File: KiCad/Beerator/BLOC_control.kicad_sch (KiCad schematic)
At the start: 10 parts, among them Y301 16MHz

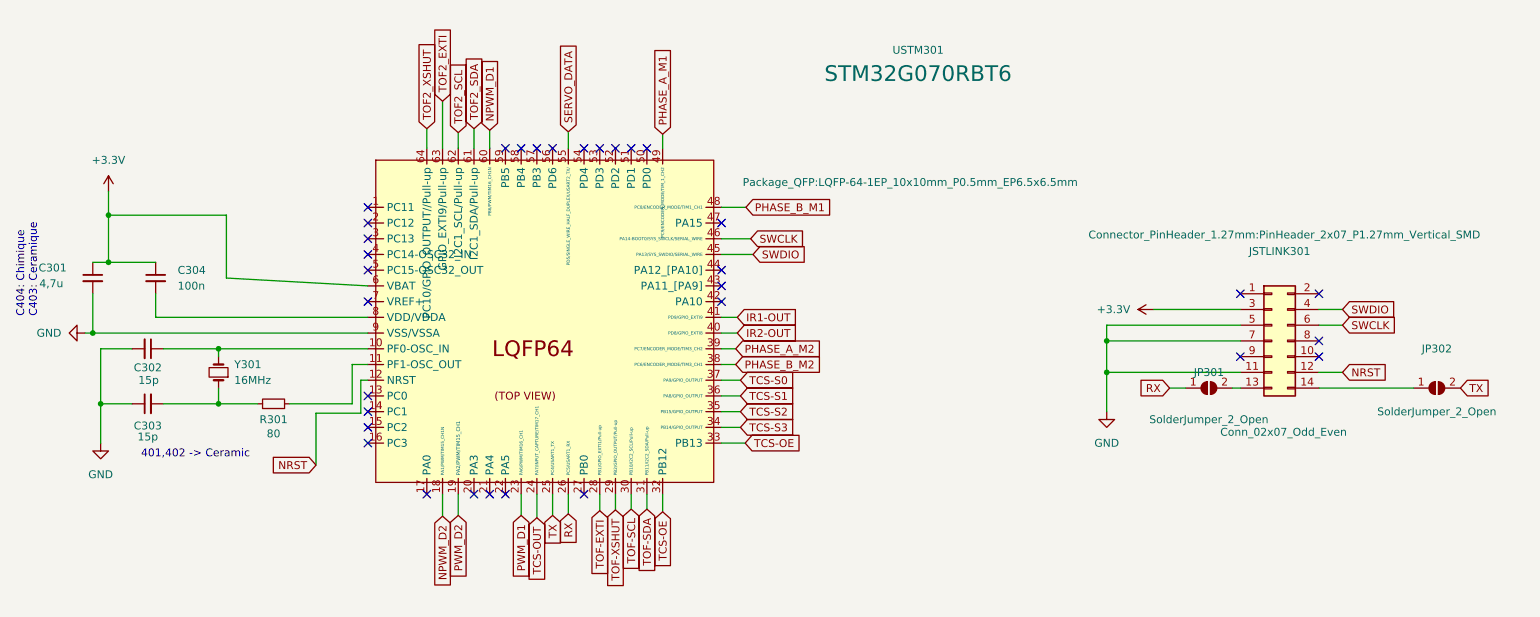
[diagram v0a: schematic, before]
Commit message: pcb_v2
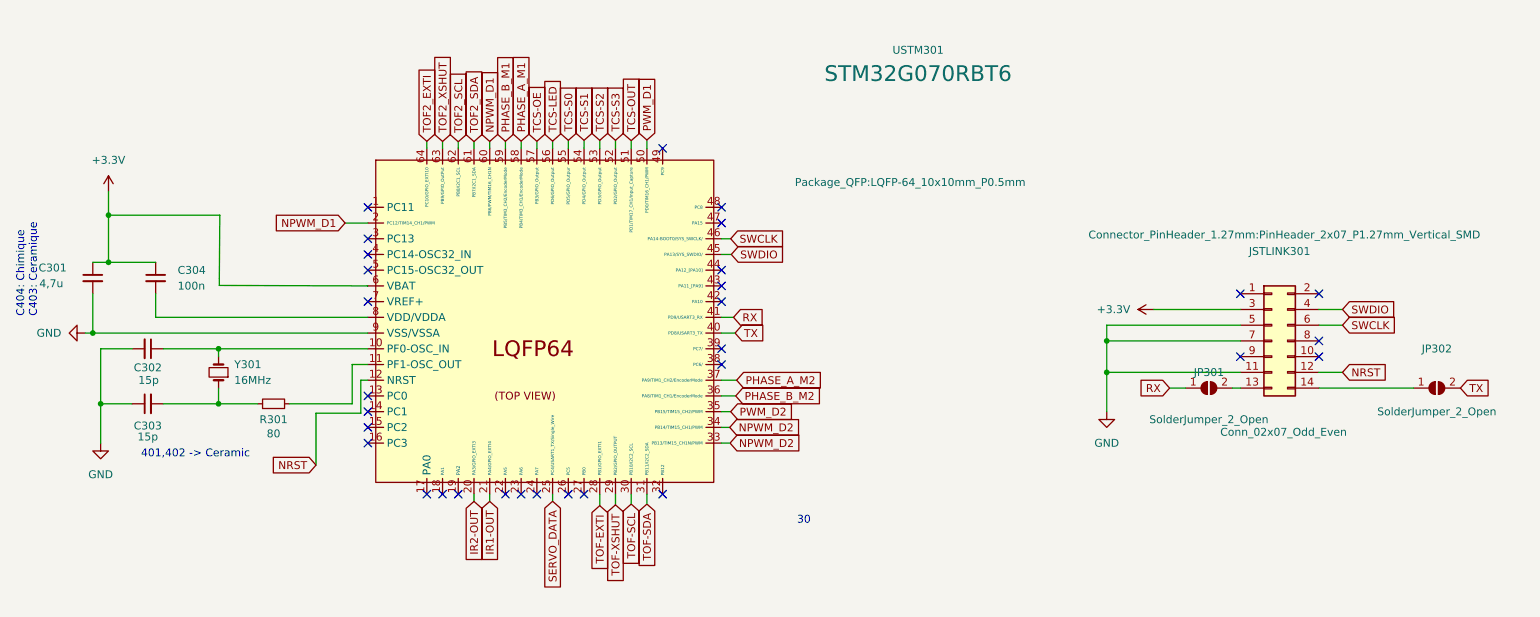
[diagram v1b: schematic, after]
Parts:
- USTM301: footprint Package_QFP:LQFP-64-1EP_10x10mm_P0.5mm_EP6.5x6.5mm -> Package_QFP:LQFP-64_10x10mm_P0.5mm
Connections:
- net IR1-OUT: now also USTM301.21 (PA4/GPIO_EXTI4); no longer USTM301.41 (PD9/GPIO_EXTI9)
- net IR2-OUT: now also USTM301.20 (PA3/GPIO_EXTI3); no longer USTM301.40 (PD8/GPIO_EXTI8)
- net NPWM_D1: now also USTM301.2 (PC12/TIM14_CH1/PWM)
- net NPWM_D2: now also USTM301.33 (PB13/TIM15_CH1N/PWM), USTM301.34 (PB14/TIM15_CH1/PWM); no longer USTM301.18 (PA1/PWM/TIM15_CH1N)
- net PHASE_A_M1: now also USTM301.58 (PB4/TIM3_CH1/EncoderMode); no longer USTM301.49 (PC9/ENCODER_MODE/TIM_1_CH2)
- net PHASE_A_M2: now also USTM301.37 (PA9/TIM1_CH2/EncoderMode); no longer USTM301.39 (PC7/ENCODER_MODE/TIM3_CH2)
- net PHASE_B_M1: now also USTM301.59 (PB5/TIM3_CH2/EncoderMode); no longer USTM301.48 (PC8/ENCODER_MODE/TIM1_CH1)
- net PHASE_B_M2: now also USTM301.36 (PA8/TIM1_CH1/EncoderMode); no longer USTM301.38 (PC6/ENCODER_MODE/TIM3_CH1)
- net PWM_D1: now also USTM301.50 (PD0/TIM16_CH1/PWM); no longer USTM301.23 (PA6/PWM/TIM16_CH1)
- net PWM_D2: now also USTM301.35 (PB15/TIM15_CH2/PWM); no longer USTM301.19 (PA2/PWM/TIM15_CH1)
- net RX: now also USTM301.41 (PD9/USART3_RX); no longer USTM301.26 (PC5/USART1_RX)
- net SERVO_DATA: now also USTM301.25 (PC4/USART1_TX/Single_Wire); no longer USTM301.55 (PD5/SINGLE_WIRE_HALF_DUPLEX/USART2_TX/)
- net TCS-OE: now also USTM301.57 (PB3/GPIO_Output); no longer USTM301.32 (PB12), USTM301.33 (PB13)
- net TCS-OUT: now also USTM301.51 (PD1/TIM17_CH1/Input_Capture); no longer USTM301.24 (PA7/INPUT_CAPTURE/TIM17_CH1)
- net TCS-S0: now also USTM301.55 (PD5/GPIO_Outpur); no longer USTM301.37 (PA9/GPIO_OUTPUT)
- net TCS-S1: now also USTM301.54 (PD4/GPIO_Output); no longer USTM301.36 (PA8/GPIO_OUTPUT)
- net TCS-S2: now also USTM301.53 (PD3/GPIO_Output); no longer USTM301.35 (PB15/GPIO_OUTPUT)
- net TCS-S3: now also USTM301.52 (PD2/GPIO_Output); no longer USTM301.34 (PB14/GPIO_OUTPUT)
- net TOF2_EXTI: now also USTM301.64 (PC10/GPIO_EXTI10); no longer USTM301.63 (GPIO_EXTI9/Pull-up)
- net TOF2_XSHUT: now also USTM301.63 (PB9/GPIO_OutPut); no longer USTM301.64 (PC10/GPIO_OUTPUT//Pull-up)
- net TX: now also USTM301.40 (PD8/USART3_TX); no longer USTM301.25 (PC4/USART1_TX)
- net TCS-LED: now reaches USTM301.56 (PD6/GPIO_Output)
- no-connect marks 33 -> 31
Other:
- note added: "30"

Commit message: version_finale_pcb
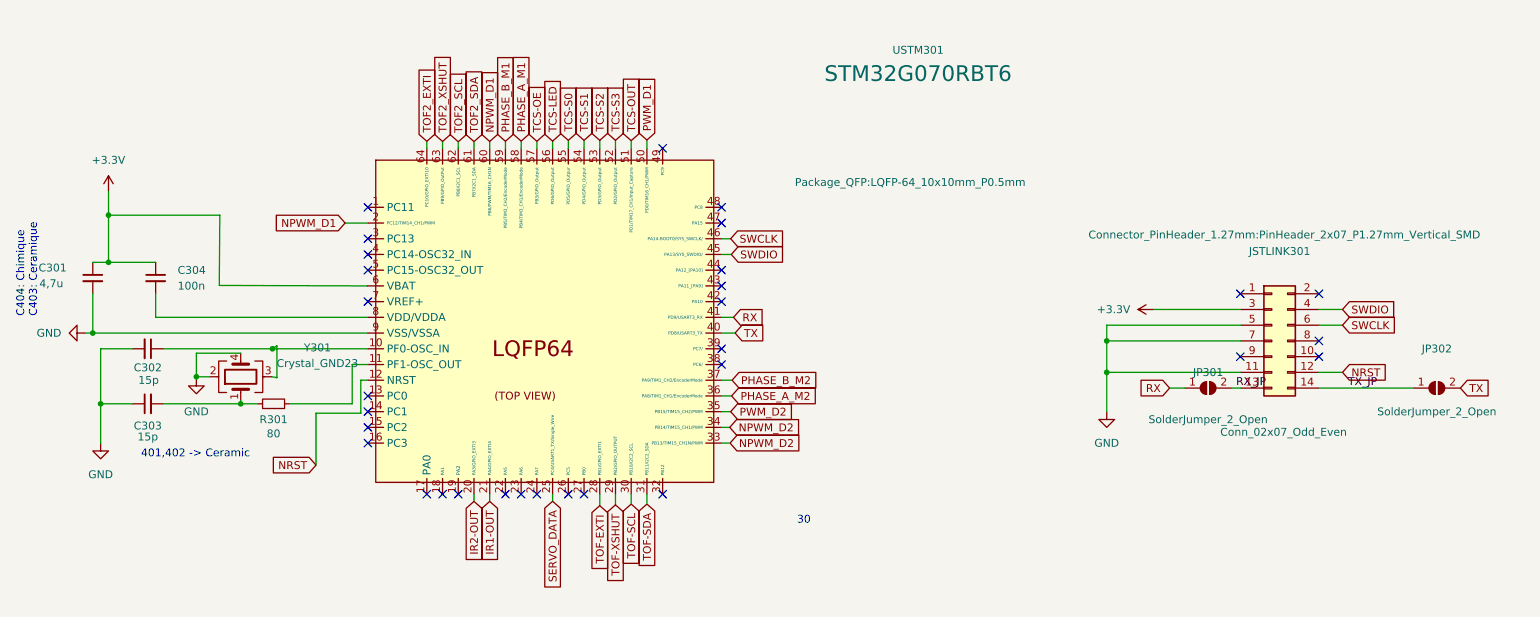
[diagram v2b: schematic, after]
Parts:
- removed Y301: 16MHz, Crystal:Crystal_SMD_0603-4Pin_6.0x3.5mm, symbol Device:Crystal_Small
- added Y301: Crystal_GND23, Crystal:Crystal_SMD_EuroQuartz_MT-4Pin_3.2x2.5mm, symbol Device:Crystal_GND23
- JP301, JP302: footprint Jumper:SolderJumper-3_P2.0mm_Open_TrianglePad1.0x1.5mm -> Jumper:SolderJumper-2_P1.3mm_Open_Pad1.0x1.5mm
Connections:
- net GND: now also Y301.2, Y301.4
- net PHASE_A_M2: now also USTM301.36 (PA8/TIM1_CH1/EncoderMode); no longer USTM301.37 (PA9/TIM1_CH2/EncoderMode)
- net PHASE_B_M2: now also USTM301.37 (PA9/TIM1_CH2/EncoderMode); no longer USTM301.36 (PA8/TIM1_CH1/EncoderMode)
- net at C302.1, USTM301.10 (PF0-OSC_IN): now also Y301.3
- net at C303.2, R301.1: now also Y301.1
- net TX_JP: now reaches JP302.1 (A), JSTLINK301.14 (Pin_14)
- net RX_JP: now reaches JP301.2 (B), JSTLINK301.13 (Pin_13)
